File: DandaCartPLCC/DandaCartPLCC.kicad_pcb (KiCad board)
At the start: 2 copper layers, 46.5 x 32 mm, 3 parts, among them P1 DAN_CART_EDGE, U1 SST39SF040

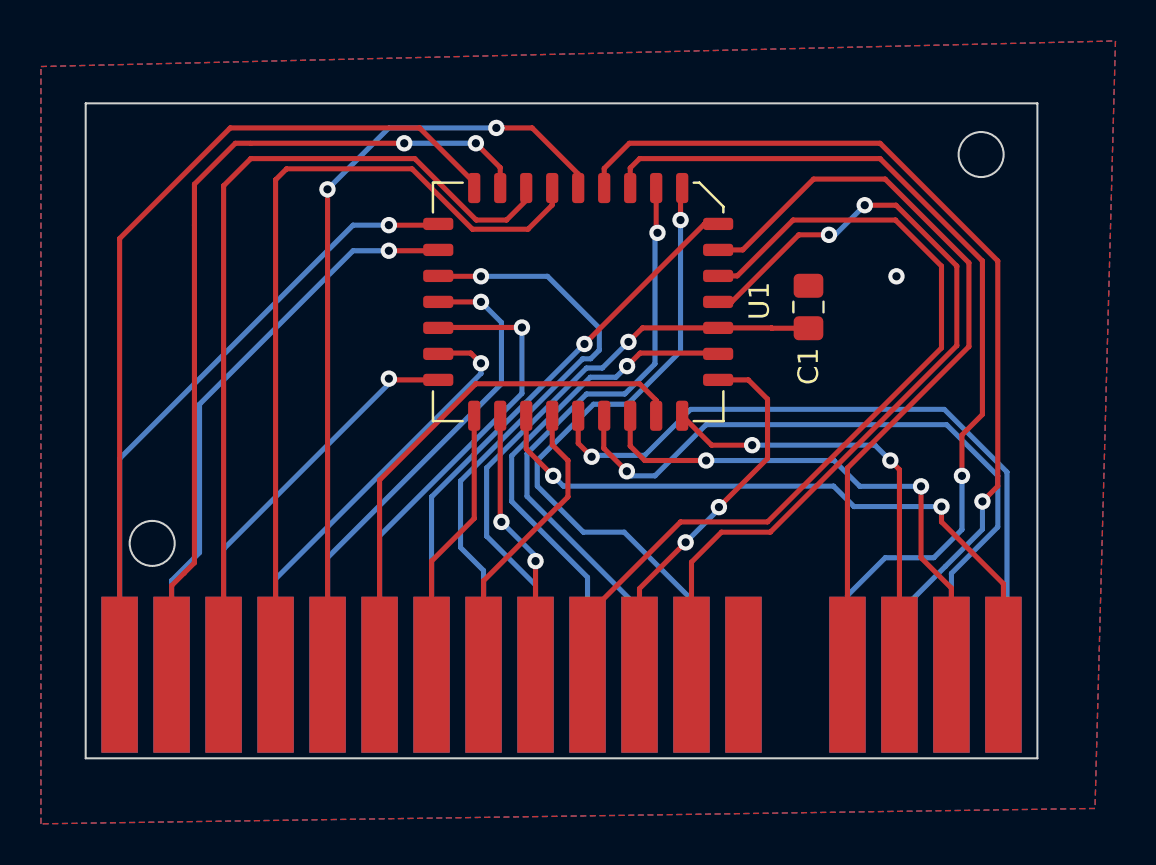
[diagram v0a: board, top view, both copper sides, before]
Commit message: Add files via upload
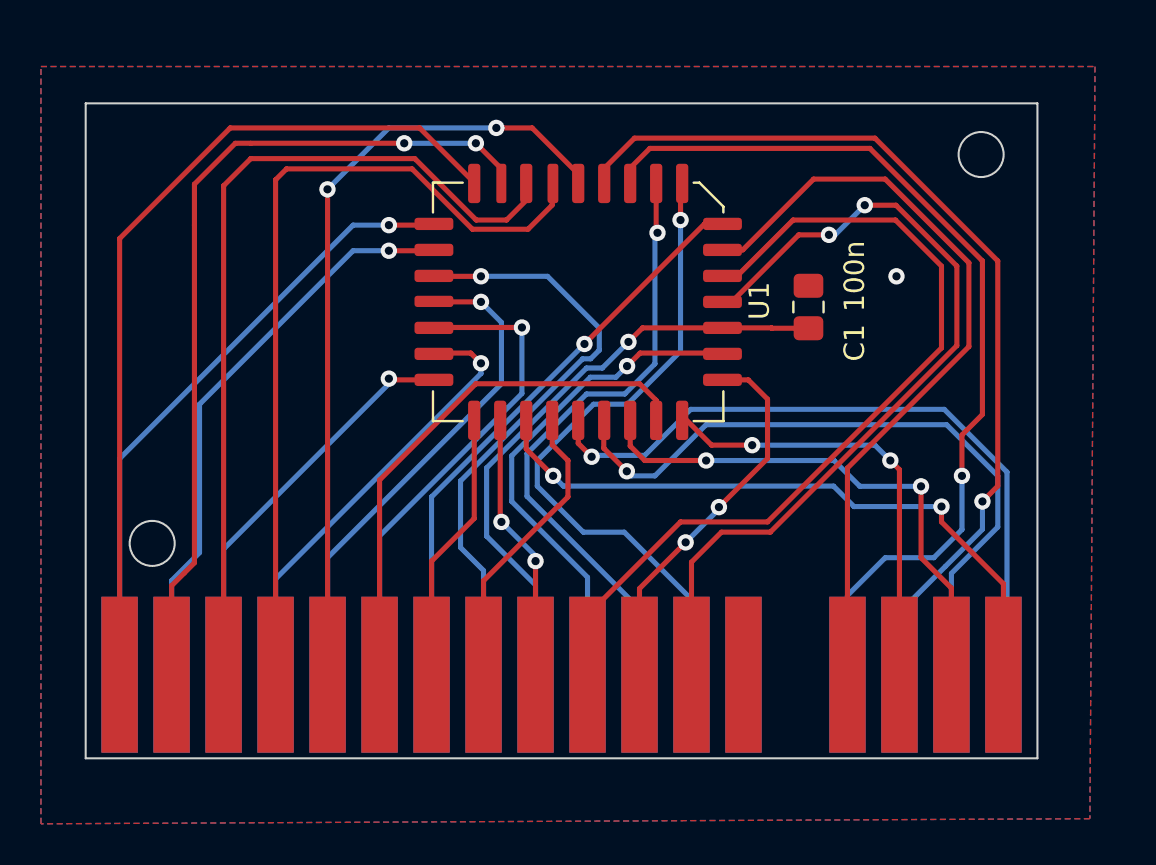
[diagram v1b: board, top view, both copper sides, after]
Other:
- board text added: "100n"
